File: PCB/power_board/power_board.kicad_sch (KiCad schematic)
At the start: 45 parts, among them IC7 BQ51013BRHLR, IC9 MAX17048G+T10, J10 Conn_01x15, J11 Conn_01x15, J7 Conn_01x02, J8 UJ20-C-H-G-MSMT-R-4C-P16-TR, Q2 Si2323DDS-T1-GE3, U2 MCP73871-2CA

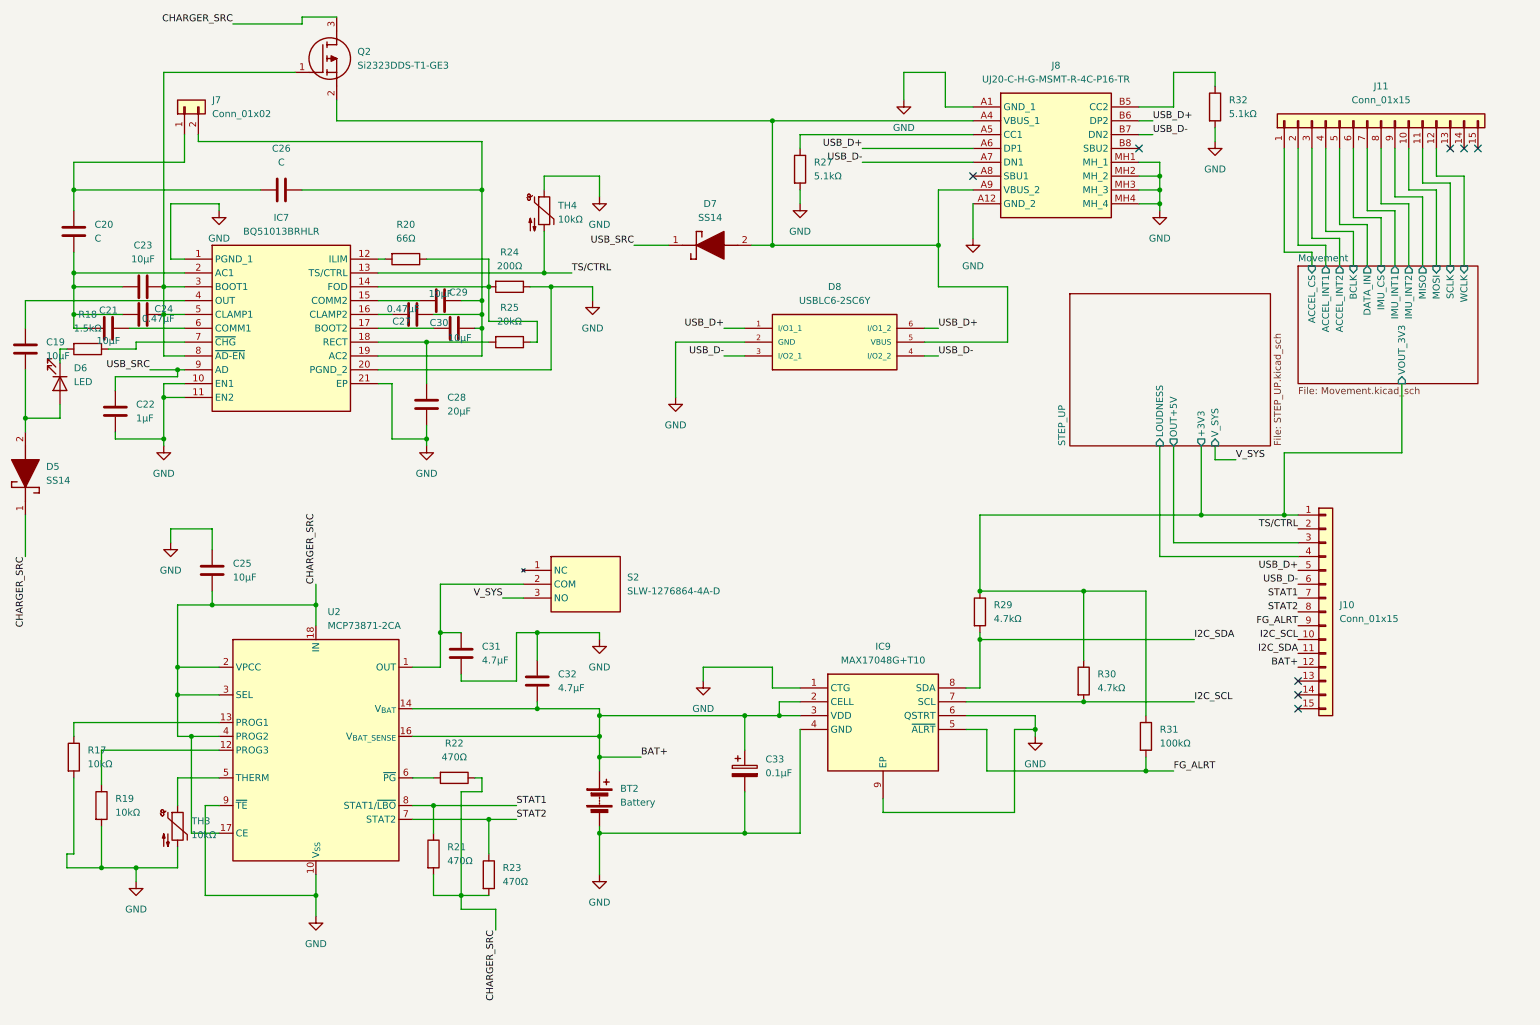
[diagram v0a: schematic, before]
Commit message: everything before jlc template
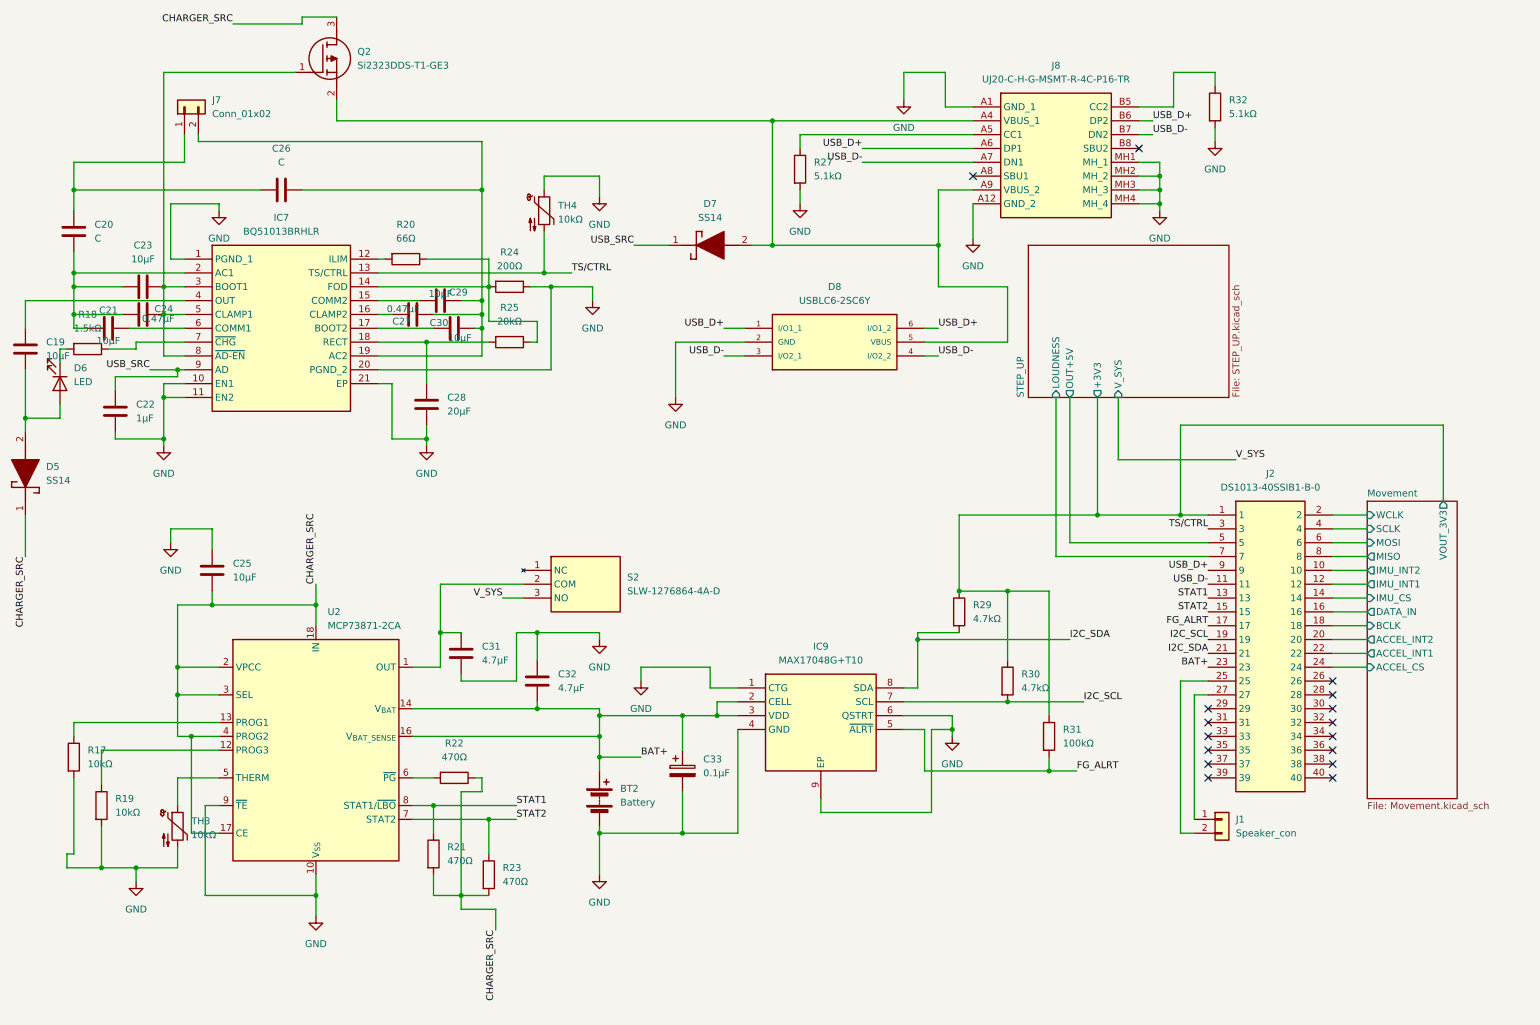
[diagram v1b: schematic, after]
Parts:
- removed J10, J11: Conn_01x15, Connector_PinHeader_2.54mm:PinHeader_1x15_P2.54mm_Vertical, symbol Connector_Generic:Conn_01x15
- added J1: Speaker_con, Connector_PinHeader_2.54mm:PinHeader_1x02_P2.54mm_Vertical, symbol Connector_Generic:Conn_01x02
- added J2: DS1013-40SSIB1-B-0, DS1013-40SSIB1-B-0:DS101340SSIB1B0, symbol DS1013-40SSIB1-B-0:DS1013-40SSIB1-B-0
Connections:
- net BAT+: now also J2.23
- net FG_ALRT: now also J2.17
- net I2C_SCL: now also J2.19
- net I2C_SDA: now also J2.21
- net Movement/ACCEL_CS: now also J2.24
- net Movement/ACCEL_INT1: now also J2.22
- net Movement/ACCEL_INT2: now also J2.20
- net Movement/BCLK: now also J2.18
- net Movement/DATA_IN: now also J2.16
- net Movement/IMU_CS: now also J2.14
- net Movement/IMU_INT1: now also J2.12
- net Movement/IMU_INT2: now also J2.10
- net Movement/MISO: now also J2.8
- net Movement/MOSI: now also J2.6
- net Movement/SCLK: now also J2.4
- net Movement/VOUT_3V3: now also J2.1
- net Movement/WCLK: now also J2.2
- net STAT1: now also J2.13
- net STAT2: now also J2.15
- net STEP_UP/LOUDNESS: now also J2.7
- net STEP_UP/OUT+5V: now also J2.5
- net TS/CTRL: now also J2.3
- net USB_D+: now also J2.9
- net USB_D-: now also J2.11
- new net: J1.1 (Pin_1), J2.27
- new net: J1.2 (Pin_2), J2.25
- no-connect marks 8 -> 16
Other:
- moved on the sheet: C33, IC9, R29, R30, R31
